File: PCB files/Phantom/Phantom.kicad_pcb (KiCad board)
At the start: 2 copper layers, 6 parts, among them J1 MEM2052-00-195-00-A_REVA, U1 ESP32-S3-MINI-1, U2 MAX-M10S, U3 D3V3XA4B10LP, U5 TLV76733DRVx, U6 MCP73871-2CC

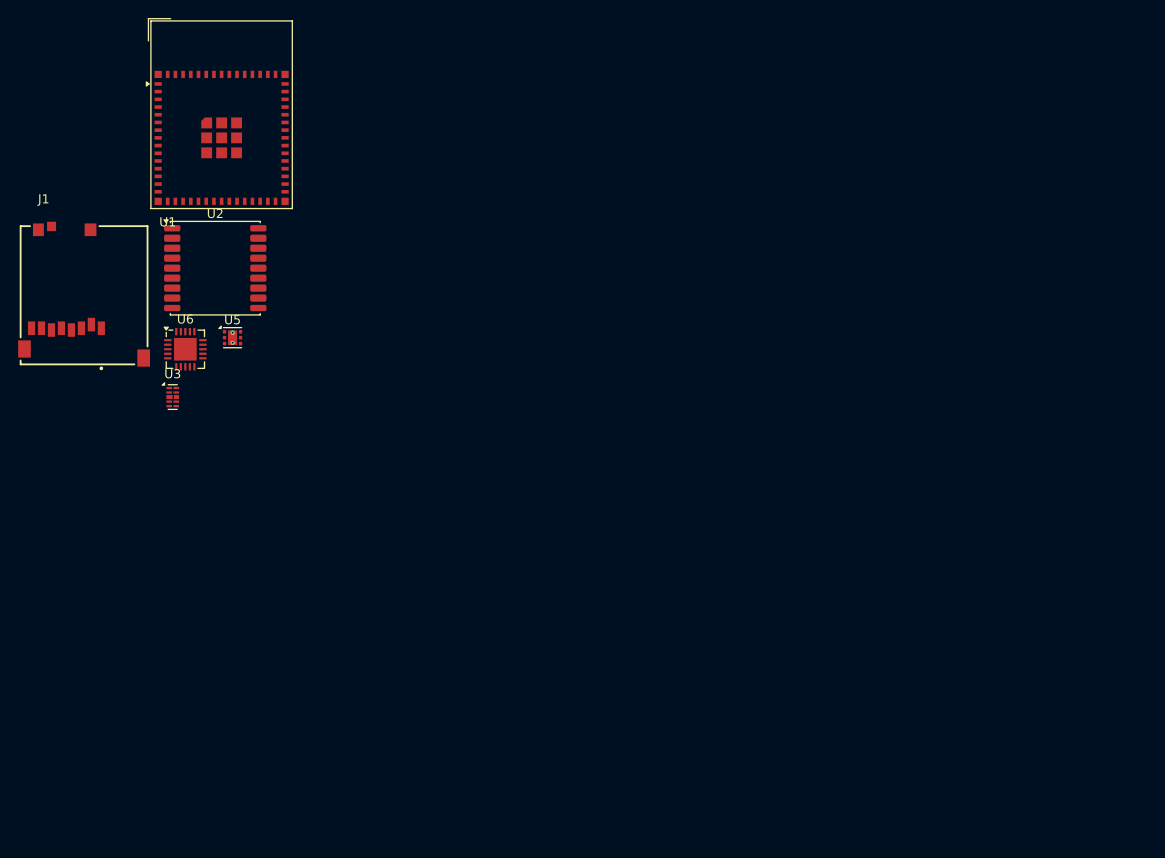
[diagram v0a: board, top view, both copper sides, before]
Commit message: Finished PCB and starting CAD
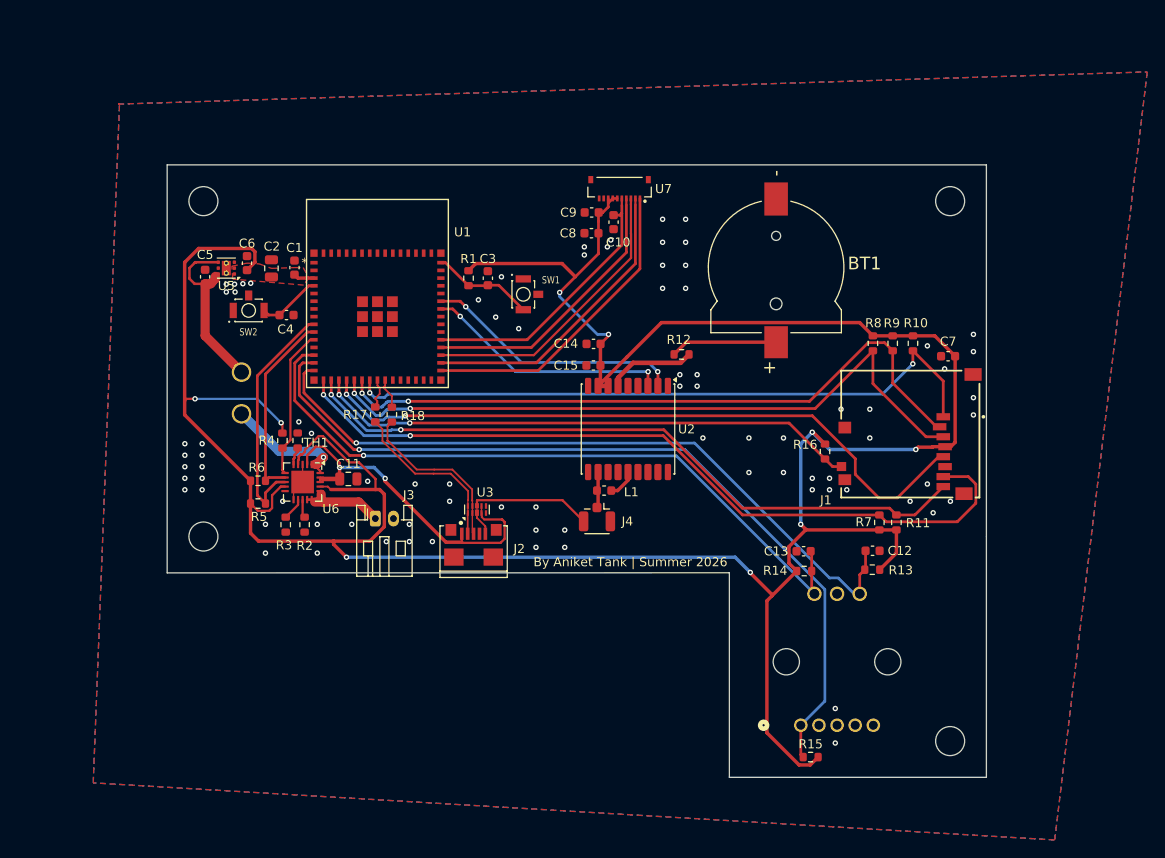
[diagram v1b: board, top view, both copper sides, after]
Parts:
- added BT1: Battery_Cell, BC501SM:BAT_BC501SM, F.Cu at (177.0, 98.0)
- added C1: 100n, Capacitor_SMD:C_0603_1608Metric, F.Cu at (123.9, 98.0)
- added C10: 100n, Capacitor_SMD:C_0603_1608Metric, F.Cu at (159.1, 93.0)
- added C11: 10u, Capacitor_SMD:C_0805_2012Metric, F.Cu at (129.8, 121.4)
- added C12: 100n, Capacitor_SMD:C_0603_1608Metric, F.Cu at (187.6, 129.3)
- added C13: 100n, Capacitor_SMD:C_0603_1608Metric, F.Cu at (180.0, 129.3)
- added C14: 2.2u, Capacitor_SMD:C_0603_1608Metric, F.Cu at (156.8, 106.5)
- added C15: 100n, Capacitor_SMD:C_0603_1608Metric, F.Cu at (156.8, 108.8)
- added C2: 22u, Capacitor_SMD:C_0805_2012Metric, F.Cu at (121.3, 98.1)
- added C3: 100n, Capacitor_SMD:C_0603_1608Metric, F.Cu at (145.2, 99.2)
- added C4: 100n, Capacitor_SMD:C_0603_1608Metric, F.Cu at (123.0, 103.3)
- added C5: 1u, Capacitor_SMD:C_0603_1608Metric, F.Cu at (114.0, 99.1)
- added C6: 2.2u, Capacitor_SMD:C_0603_1608Metric, F.Cu at (118.6, 97.5)
- added C7: 100n, Capacitor_SMD:C_0603_1608Metric, F.Cu at (196.0, 107.8)
- added C8: 100n, Capacitor_SMD:C_0603_1608Metric, F.Cu at (156.6, 94.2)
- added C9: 1u, Capacitor_SMD:C_0603_1608Metric, F.Cu at (156.6, 92.0)
- added H1: MountingHole, MountingHole:MountingHole_3.2mm_M3, F.Cu at (196.1, 90.7)
- added H2: MountingHole, MountingHole:MountingHole_3.2mm_M3, F.Cu at (113.8, 127.7)
- added H3: MountingHole, MountingHole:MountingHole_3.2mm_M3, F.Cu at (113.8, 90.7)
- added H4: MountingHole, MountingHole:MountingHole_3.2mm_M3, F.Cu at (196.2, 150.3)
- added J2: USB_B_Micro, DX4R005HJ5R2000:JAE_DX4R005HJ5R2000, F.Cu at (143.6, 127.4)
- added J3: Conn_01x02_Socket, Connector_JST:JST_PH_S2B-PH-K_1x02_P2.00mm_Horizontal, F.Cu at (132.8, 125.7)
- added J4: Conn_Coaxial, Connector_Coaxial:U.FL_Hirose_U.FL-R-SMT-1_Vertical, F.Cu at (157.2, 125.6)
- added L1: 47n, Inductor_SMD:L_0603_1608Metric, F.Cu at (158.0, 122.6)
- added R1: 10k, Resistor_SMD:R_0603_1608Metric, F.Cu at (143.1, 99.2)
- added R10: 10k, Resistor_SMD:R_0603_1608Metric, F.Cu at (192.1, 106.4)
- added R11: 10k, Resistor_SMD:R_0603_1608Metric, F.Cu at (190.3, 126.2)
- added R12: 10, Resistor_SMD:R_0603_1608Metric, F.Cu at (166.6, 107.6)
- added R13: 10k, Resistor_SMD:R_0603_1608Metric, F.Cu at (187.6, 131.4)
- added R14: 10k, Resistor_SMD:R_0603_1608Metric, F.Cu at (180.1, 131.5)
- added R15: 10k, Resistor_SMD:R_0603_1608Metric, F.Cu at (180.8, 152.0)
- added R16: 10k, Resistor_SMD:R_0603_1608Metric, F.Cu at (182.4, 118.3)
- added R17: 0, Resistor_SMD:R_0603_1608Metric, F.Cu at (132.8, 114.2)
- added R18: 0, Resistor_SMD:R_0603_1608Metric, F.Cu at (134.6, 114.3)
- added R2: 2k, Resistor_SMD:R_0603_1608Metric, F.Cu at (125.0, 126.4)
- added R3: 20k, Resistor_SMD:R_0603_1608Metric, F.Cu at (122.9, 126.4)
- added R4: 10k, Resistor_SMD:R_0603_1608Metric, F.Cu at (122.5, 117.1)
- added R5: 10k, Resistor_SMD:R_0603_1608Metric, F.Cu at (119.8, 124.1)
- added R6: 10k, Resistor_SMD:R_0603_1608Metric, F.Cu at (119.8, 121.6)
- added R7: 10k, Resistor_SMD:R_0603_1608Metric, F.Cu at (188.4, 126.2)
- added R8: 10k, Resistor_SMD:R_0603_1608Metric, F.Cu at (187.7, 106.4)
- added R9: 10k, Resistor_SMD:R_0603_1608Metric, F.Cu at (189.9, 106.4)
- added SW1: SW_Push, B3U_1100P:SW_B3U-1100P, F.Cu at (149.1, 101.0)
- added SW2: SW_Push, B3U_1100P:SW_B3U-1100P, F.Cu at (118.8, 102.8)
- added SW3: RotaryEncoder_Switch, footprintsconn:COM-15141_SPK, B.Cu at (179.7, 148.5)
- added SW4: SW_SPST, footprintsSPST:SW_1MS02Q_CNK, B.Cu at (118.0, 109.6)
- added TH1: Thermistor_NTC, Resistor_SMD:R_0603_1608Metric, F.Cu at (124.2, 117.1)
- added U7: ~, FH33_10S_0_5SH_10_:HRS_FH33-10S-0.5SH_10_, F.Cu at (159.7, 90.4)
- U1: footprint RF_Module:ESP32-S2-MINI-1 -> foot:ESP32-S3-MINI-1_EXP
- moved J1 92.4 mm to (191.8, 116.4), turned to 90 degrees
- moved U2 48.9 mm to (160.6, 115.8), turned to -90 degrees
- moved U3 35.8 mm to (144.0, 124.7), turned to 90 degrees
- moved U1 26.2 mm to (133.0, 100.9)
- moved U6 19.5 mm to (124.7, 121.7), turned to -90 degrees
- moved U5 7.71 mm to (116.3, 98.1), turned to 180 degrees
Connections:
- U1 pad 10: /DAT2 -> /STAT2
- U1 pad 11: /DAT3 -> /PG
- U1 pad 12: /CD_PIN -> unconnected-(U1-IO8-Pad12)
- U1 pad 13: unconnected-(U1-IO9-Pad13) -> /A
- U1 pad 14: unconnected-(U1-IO10-Pad14) -> /S1
- U1 pad 15: unconnected-(U1-IO11-Pad15) -> /B
- U1 pad 16: unconnected-(U1-IO12-Pad16) -> /DAT0
- U1 pad 17: unconnected-(U1-IO13-Pad17) -> /DAT1
- U1 pad 18: unconnected-(U1-IO14-Pad18) -> /CD_PIN
- U1 pad 19: unconnected-(U1-IO15-Pad19) -> /CLK
- U1 pad 20: unconnected-(U1-IO16-Pad20) -> /CMD
- U1 pad 21: unconnected-(U1-IO17-Pad21) -> /DAT3
- U1 pad 22: unconnected-(U1-IO18-Pad22) -> /DAT2
- U1 pad 23: /D- -> /1D-
- U1 pad 24: /D+ -> /2D+
- U1 pad 26: /SCS -> unconnected-(U1-IO26-Pad26)
- U1 pad 27: /PG -> unconnected-(U1-IO47-Pad27)
- U1 pad 28: /SI -> unconnected-(U1-IO33-Pad28)
- U1 pad 29: /SCLK -> unconnected-(U1-IO34-Pad29)
- U1 pad 31: unconnected-(U1-IO35-Pad31) -> /SCLK
- U1 pad 32: unconnected-(U1-IO36-Pad32) -> /SI
- U1 pad 33: unconnected-(U1-IO37-Pad33) -> /SCS
- U1 pad 35: unconnected-(U1-IO39-Pad35) -> /DISPCNTRL
- U1 pad 37: /STAT1 -> unconnected-(U1-IO41-Pad37)
- U1 pad 39: unconnected-(U1-TXD0-Pad39) -> /GPSRX
- U1 pad 40: unconnected-(U1-RXD0-Pad40) -> /GPSTX
- U1 pad 41: /STAT2 -> unconnected-(U1-IO45-Pad41)
- U1 pad 5: /CLK -> unconnected-(U1-IO1-Pad5)
- U1 pad 6: /CMD -> unconnected-(U1-IO2-Pad6)
- U1 pad 8: /DAT0 -> unconnected-(U1-IO4-Pad8)
- U1 pad 9: /DAT1 -> /STAT1
- U2 pad 11: unconnected-(U2-RF_IN-Pad11) -> Net-(J4-In)
- U2 pad 14: unconnected-(U2-VCC_RF-Pad14) -> Net-(U2-VCC_RF)
- U2 pad 6: unconnected-(U2-V_BCKP-Pad6) -> /VBCK
- U6 pad 1: /LDOIN -> /OUT
- U6 pad 20: /LDOIN -> /OUT
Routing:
- net +3.3V: track 0.00 -> 329.5 mm, vias 0 -> 9
- net /S1: track 0.00 -> 91.5 mm, vias 0 -> 1
- net /DAT0: track 0.00 -> 86.3 mm, vias 0 -> 2
- net /B: track 0.00 -> 78.9 mm, vias 0 -> 1
- net /A: track 0.00 -> 77.7 mm, vias 0 -> 1
- net /CMD: track 0.00 -> 76.8 mm, vias 0 -> 2
- net /DAT1: track 0.00 -> 76.3 mm, vias 0 -> 2
- net /CLK: track 0.00 -> 75.5 mm, vias 0 -> 2
- net /DAT3: track 0.00 -> 74.8 mm, vias 0 -> 2
- net /DAT2: track 0.00 -> 73.3 mm, vias 0 -> 2
- net /CD_PIN: track 0.00 -> 60.6 mm, vias 0 -> 2
- net /VBUS: track 0.00 -> 38.7 mm, vias 0 -> 2
- net /SCLK: track 0.00 -> 34.4 mm
- net /SI: track 0.00 -> 33.2 mm
- net /SCS: track 0.00 -> 32.0 mm
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- added copper zone on F.Cu, net +3.3V
- added copper zone on B.Cu, net GND
- added copper zone on F.Cu, net GND
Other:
- board outline added: 90.4 x 67.6 mm
- board text added: "By Aniket Tank | Summer 2026"
